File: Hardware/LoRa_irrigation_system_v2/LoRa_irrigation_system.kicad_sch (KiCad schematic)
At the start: 14 parts, among them J1 12VIN, J2 SoilMoisture sensor, J3 WaterPump connector, J4 Conn_Coaxial, K2 SANYOU_SRD_Form_C, U1 LM2596_buck_converter, U2 RASPBERRY_PI_PICO, U4 RFM69HCW LoRa module

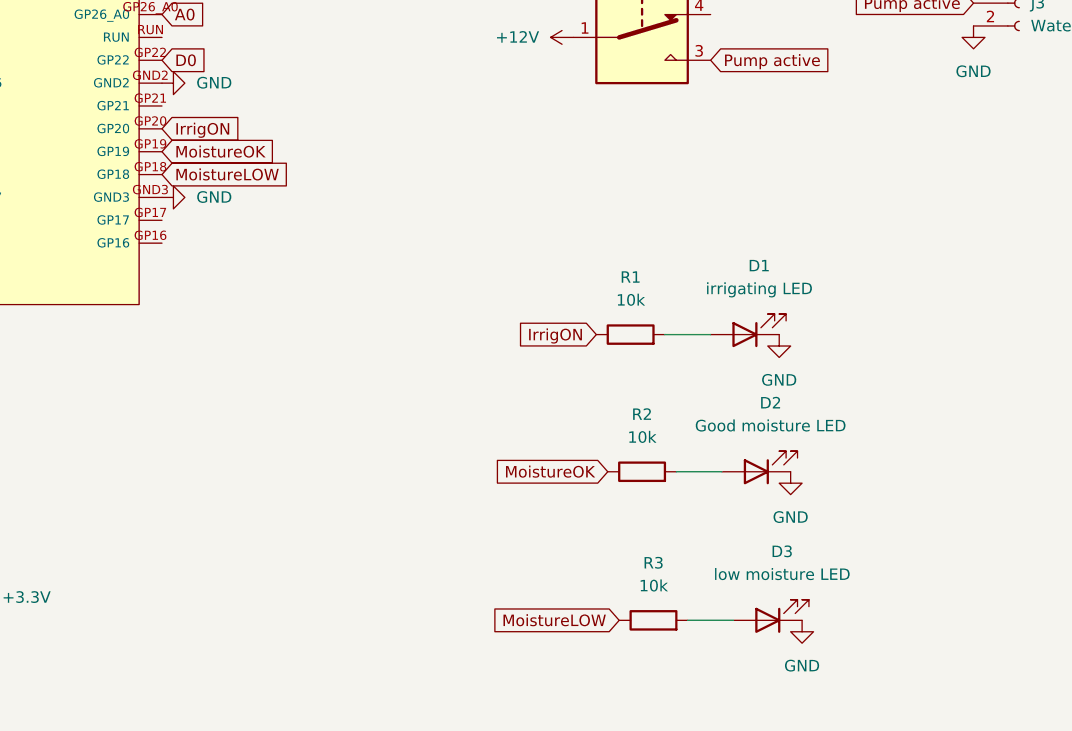
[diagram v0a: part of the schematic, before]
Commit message: updated hardware
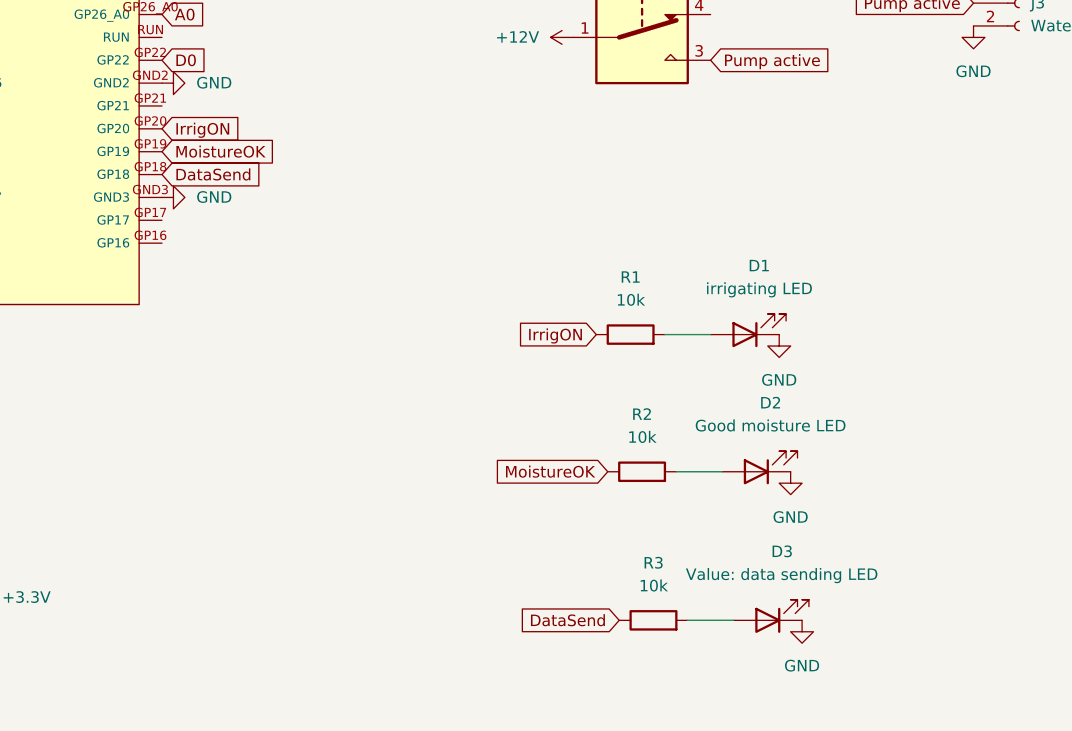
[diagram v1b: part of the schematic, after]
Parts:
- D3: value low moisture LED -> data sending LED
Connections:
- net MoistureLOW renamed DataSend
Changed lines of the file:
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@@
 		)
 	)
-	(global_label "MoistureLOW"
+	(global_label "SCK"
 		(shape input)
-		(at 187.96 144.78 180)
+		(at 111.76 62.23 180)
 		(fields_autoplaced yes)
 		(effects
@@
 		)
 		(property "Intersheetrefs" "${INTERSHEET_REFS}"
-			(at 173.182 144.78 0)
+			(at 105.0253 62.23 0)
 			(effects
 				(font
@@
 		)
 	)
-	(global_label "SCK"
+	(global_label "DIO0"
 		(shape input)
-		(at 111.76 62.23 180)
+		(at 80.01 73.66 0)
 		(fields_autoplaced yes)
 		(effects
@@
 				(size 1.27 1.27)
 			)
-			(justify right)
+			(justify left)
 		)
 		(property "Intersheetrefs" "${INTERSHEET_REFS}"
-			(at 105.0253 62.23 0)
-			(effects
-				(font
-					(size 1.27 1.27)
-				)
-				(justify right)
-				(hide yes)
-			)
-		)
-	)
-	(global_label "DIO0"
+			(at 87.41 73.66 0)
+			(effects
+				(font
+					(size 1.27 1.27)
+				)
+				(justify left)
+				(hide yes)
+			)
+		)
+	)
+	(global_label "RelayON"
 		(shape input)
-		(at 80.01 73.66 0)
+		(at 111.76 102.87 180)
 		(fields_autoplaced yes)
 		(effects
@@
 				(size 1.27 1.27)
 			)
-			(justify left)
+			(justify right)
 		)
 		(property "Intersheetrefs" "${INTERSHEET_REFS}"
-			(at 87.41 73.66 0)
-			(effects
-				(font
-					(size 1.27 1.27)
-				)
-				(justify left)
-				(hide yes)
-			)
-		)
-	)
-	(global_label "RelayON"
+			(at 100.9734 102.87 0)
+			(effects
+				(font
+					(size 1.27 1.27)
+				)
+				(justify right)
+				(hide yes)
+			)
+		)
+	)
+	(global_label "MoistureOK"
 		(shape input)
-		(at 111.76 102.87 180)
+		(at 186.69 128.27 180)
 		(fields_autoplaced yes)
 		(effects
@@
 		)
 		(property "Intersheetrefs" "${INTERSHEET_REFS}"
-			(at 100.9734 102.87 0)
+			(at 173.1215 128.27 0)
 			(effects
 				(font
@@
 		)
 	)
-	(global_label "MoistureOK"
+	(global_label "Pump active"
 		(shape input)
-		(at 186.69 128.27 180)
+		(at 227.33 76.2 180)
 		(fields_autoplaced yes)
 		(effects
@@
 		)
 		(property "Intersheetrefs" "${INTERSHEET_REFS}"
-			(at 173.1215 128.27 0)
+			(at 212.4916 76.2 0)
 			(effects
 				(font
@@
 		)
 	)
-	(global_label "Pump active"
+	(global_label "MOSI"
 		(shape input)
-		(at 227.33 76.2 180)
+		(at 49.53 81.28 180)
 		(fields_autoplaced yes)
 		(effects
@@
 		)
 		(property "Intersheetrefs" "${INTERSHEET_REFS}"
-			(at 212.4916 76.2 0)
+			(at 41.9486 81.28 0)
 			(effects
 				(font
@@
 		)
 	)
-	(global_label "MOSI"
+	(global_label "Pump active"
 		(shape input)
-		(at 49.53 81.28 180)
+		(at 198.12 82.55 0)
 		(fields_autoplaced yes)
 		(effects
@@
 				(size 1.27 1.27)
 			)
-			(justify right)
+			(justify left)
 		)
 		(property "Intersheetrefs" "${INTERSHEET_REFS}"
-			(at 41.9486 81.28 0)
-			(effects
-				(font
-					(size 1.27 1.27)
-				)
-				(justify right)
-				(hide yes)
-			)
-		)
-	)
-	(global_label "Pump active"
+			(at 212.9584 82.55 0)
+			(effects
+				(font
+					(size 1.27 1.27)
+				)
+				(justify left)
+				(hide yes)
+			)
+		)
+	)
+	(global_label "NSS"
 		(shape input)
-		(at 198.12 82.55 0)
+		(at 49.53 76.2 180)
 		(fields_autoplaced yes)
 		(effects
@@
 				(size 1.27 1.27)
 			)
-			(justify left)
+			(justify right)
 		)
 		(property "Intersheetrefs" "${INTERSHEET_REFS}"
-			(at 212.9584 82.55 0)
-			(effects
-				(font
-					(size 1.27 1.27)
-				)
-				(justify left)
-				(hide yes)
-			)
-		)
-	)
-	(global_label "NSS"
+			(at 42.7953 76.2 0)
+			(effects
+				(font
+					(size 1.27 1.27)
+				)
+				(justify right)
+				(hide yes)
+			)
+		)
+	)
+	(global_label "MOSI"
 		(shape input)
-		(at 49.53 76.2 180)
+		(at 111.76 64.77 180)
 		(fields_autoplaced yes)
 		(effects
@@
 		)
 		(property "Intersheetrefs" "${INTERSHEET_REFS}"
-			(at 42.7953 76.2 0)
+			(at 104.1786 64.77 0)
 			(effects
 				(font
@@
 		)
 	)
-	(global_label "MOSI"
+	(global_label "DataSend"
 		(shape input)
-		(at 111.76 64.77 180)
+		(at 187.96 144.78 180)
 		(fields_autoplaced yes)
 		(effects
@@
 		)
 		(property "Intersheetrefs" "${INTERSHEET_REFS}"
-			(at 104.1786 64.77 0)
+			(at 176.085 144.78 0)
 			(effects
 				(font
@@
 		)
 	)
-	(global_label "MoistureLOW"
+	(global_label "DataSend"
 		(shape input)
 		(at 137.16 95.25 0)
@@
 		)
 		(property "Intersheetrefs" "${INTERSHEET_REFS}"
-			(at 151.938 95.25 0)
+			(at 149.035 95.25 0)
 			(effects
 				(font
@@
 			)
 		)
-		(property "Value" "low moisture LED"
+		(property "Value" "data sending LED"
 			(at 206.0575 139.7 0)
-			(effects
-				(font
+			(show_name yes)
+			(effects
+				(font
